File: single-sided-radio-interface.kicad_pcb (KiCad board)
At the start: 2 copper layers, 40.5 x 28 mm, 23 parts, among them J10 USB_B_Micro, J5 PTT, J6 AUDIO_OUT, J7 AUDIO_IN, J8 SQUELCH, J9 GND, Q1 BSS138, U1 CM108AH, Y1 12M

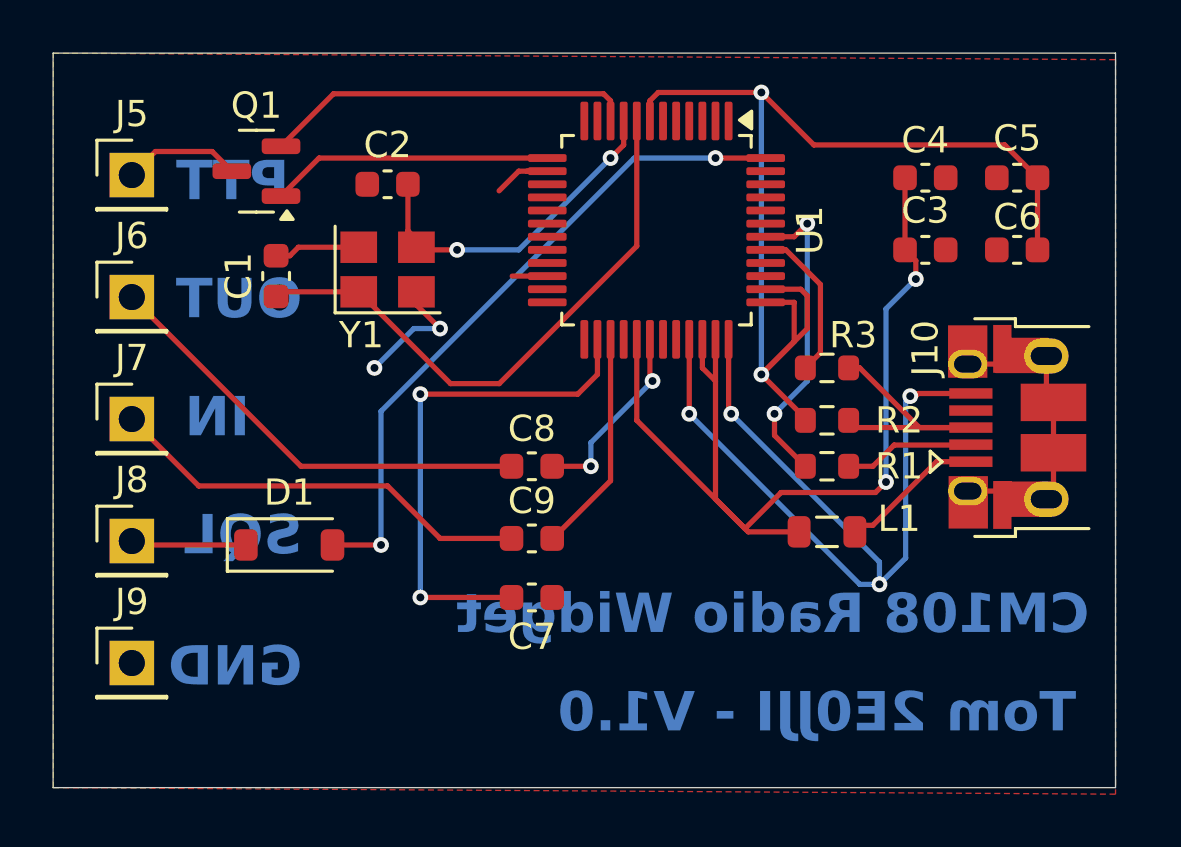
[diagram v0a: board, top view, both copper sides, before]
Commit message: V1.1 - smaller board
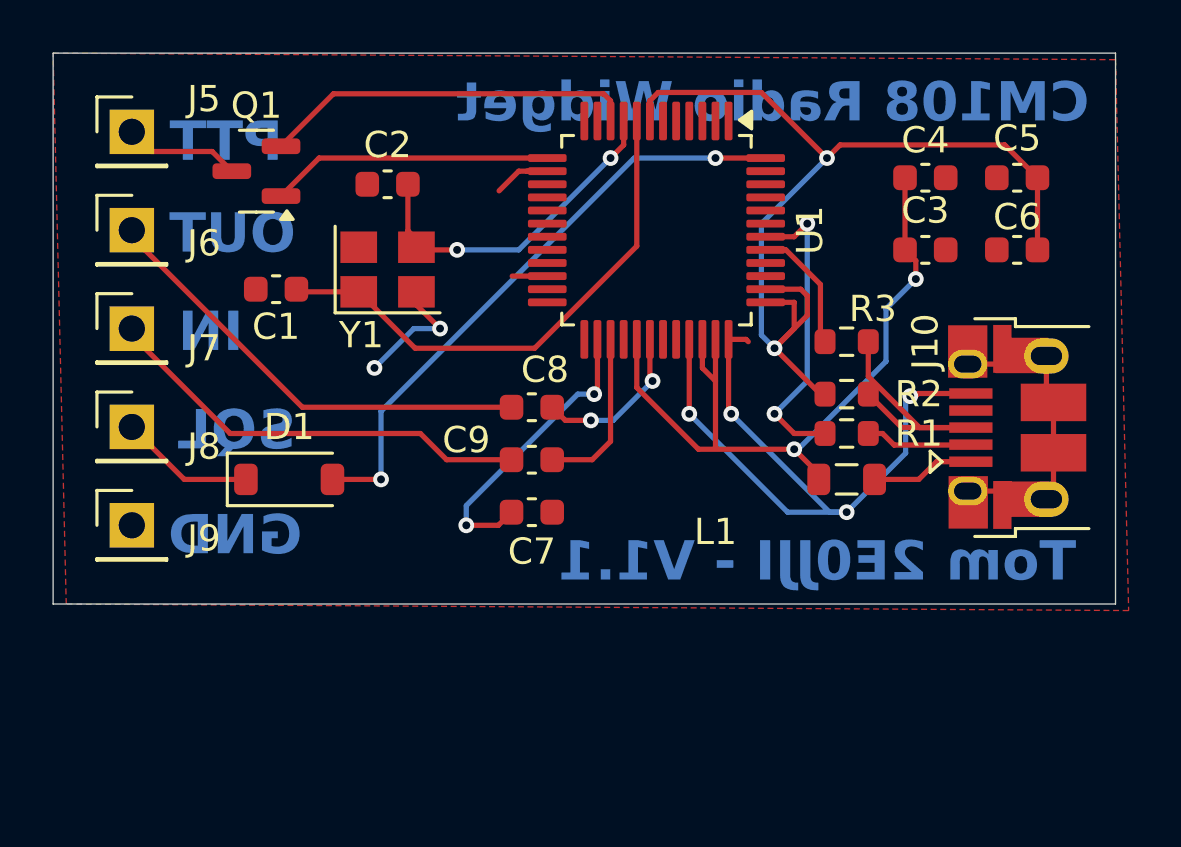
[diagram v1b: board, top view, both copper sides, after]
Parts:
- moved J9 5.25 mm to (76.0, 74.2)
- moved J8 4.35 mm to (76.0, 70.5)
- moved J7 3.45 mm to (76.0, 66.8)
- moved C7 3.25 mm to (91.2, 73.8)
- moved C9 3.00 mm to (91.2, 71.8)
- moved J6 2.55 mm to (76.0, 63.0)
- moved D1 2.50 mm to (82.0, 72.5)
- moved C8 2.25 mm to (91.2, 69.8)
- moved L1 2.14 mm to (103.2, 72.5)
- moved J5 1.65 mm to (76.0, 59.2)
- moved R1 1.46 mm to (103.2, 70.8)
- moved R2 1.25 mm to (103.2, 69.2)
- moved R3 1.25 mm to (103.2, 67.2)
- moved C1 0.50 mm to (81.5, 65.2), turned to 180 degrees
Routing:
- net GND: track 63.6 -> 53.1 mm
- net VCC: track 38.9 -> 29.1 mm
- net NET-(U1-BGREF): track 19.6 -> 11.5 mm
- net +3V3: track 42.7 -> 38.7 mm
- net Net-(D1-A): track 25.6 -> 23.1 mm
- net Net-(U1-MICIN): track 8.52 -> 6.40 mm
- net Net-(U1-XI): track 22.2 -> 20.3 mm
- net unconnected-(J10-VBUS-Pad1): track 5.53 -> 3.95 mm
- net NET-(U1-USBDP): track 6.05 -> 4.89 mm
- net Net-(U1-LOL): track 7.33 -> 6.28 mm
- net unconnected-(J10-D--Pad2): track 5.00 -> 4.10 mm
- net SQUELCH: track 4.41 -> 5.18 mm
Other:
- board size 40.5 x 28 mm -> 40.5 x 21 mm
- board text added: "Tom 2E0JJI - V1.1"
- board text removed: "Tom 2E0JJI - V1.0"
